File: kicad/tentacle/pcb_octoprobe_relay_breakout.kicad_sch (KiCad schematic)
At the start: 2 parts, among them J501 Conn_01x20, J502 Conn_01x20

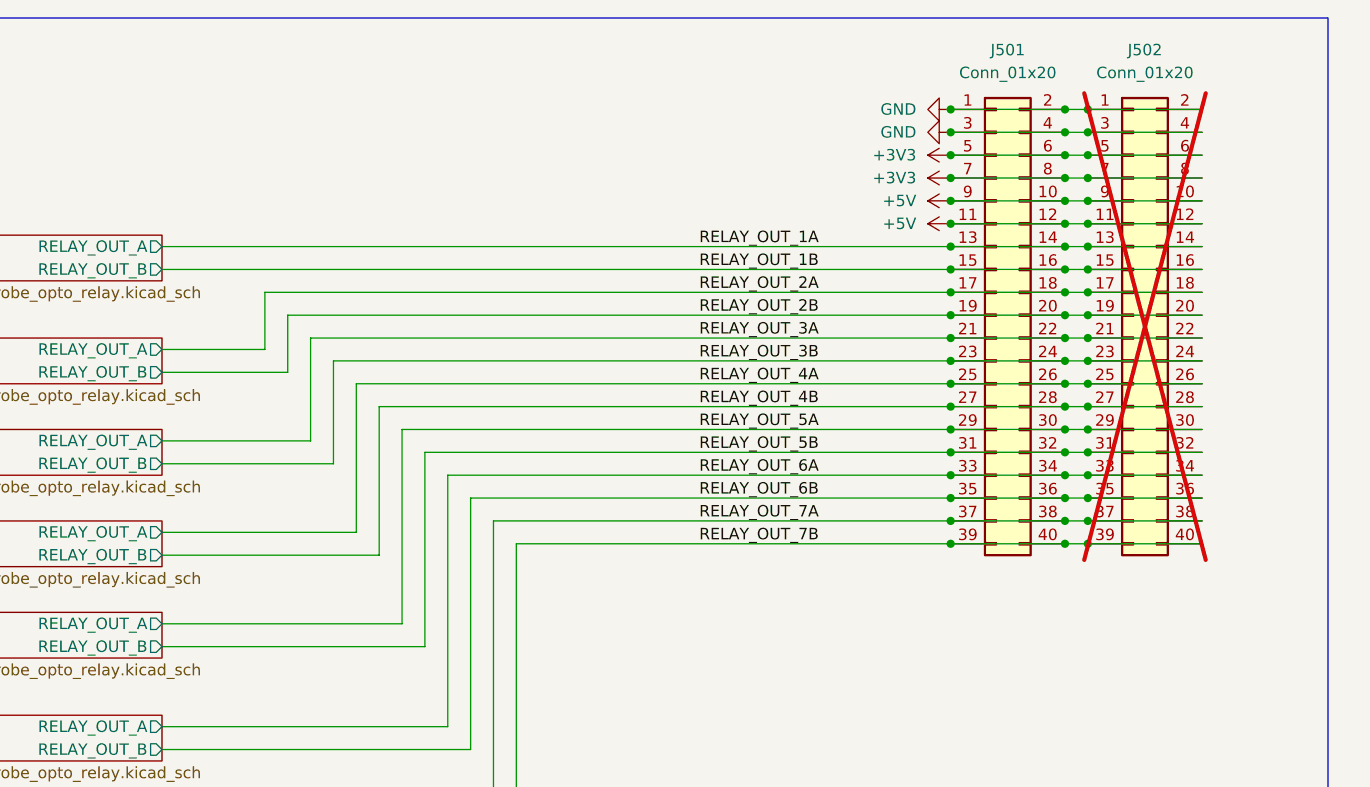
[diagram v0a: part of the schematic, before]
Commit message: Tentacle v0.4
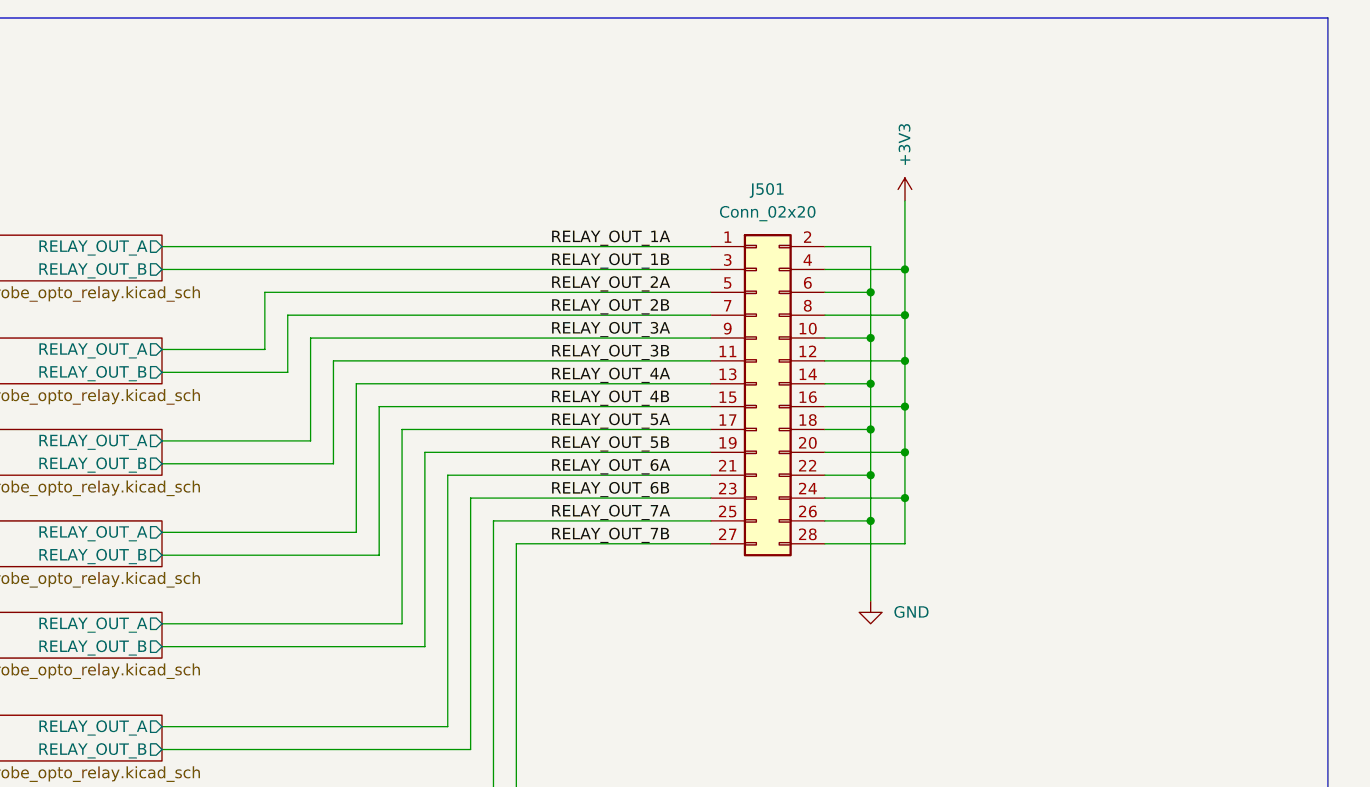
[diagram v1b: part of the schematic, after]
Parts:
- removed J501, J502: Conn_01x20, 00_project_library:PinSocket_2x20_P2.54mm_Vertical_squarepad, symbol Connector_Generic:Conn_02x20_Odd_Even
- added J501: Conn_02x20, 00_project_library:PinSocket_2x14_P2.54mm_Vertical_squarepad, symbol Connector_Generic:Conn_02x14_Odd_Even
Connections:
- net +3V3: now also J501.12 (Pin_12), J501.16 (Pin_16), J501.20 (Pin_20), J501.24 (Pin_24), J501.28 (Pin_28), J501.4 (Pin_4), J501.8 (Pin_8)
- net GND: now also J501.10 (Pin_10), J501.14 (Pin_14), J501.18 (Pin_18), J501.2 (Pin_2), J501.22 (Pin_22), J501.26 (Pin_26), J501.6 (Pin_6)
- net RELAY_OUT_1A: now also J501.1 (Pin_1)
- net RELAY_OUT_1B: now also J501.3 (Pin_3)
- net RELAY_OUT_2A: now also J501.5 (Pin_5)
- net RELAY_OUT_2B: now also J501.7 (Pin_7)
- net RELAY_OUT_3A: now also J501.9 (Pin_9)
- net RELAY_OUT_3B: now also J501.11 (Pin_11)
- net RELAY_OUT_4A: now also J501.13 (Pin_13)
- net RELAY_OUT_4B: now also J501.15 (Pin_15)
- net RELAY_OUT_5A: now also J501.17 (Pin_17)
- net RELAY_OUT_5B: now also J501.19 (Pin_19)
- net RELAY_OUT_6A: now also J501.21 (Pin_21)
- net RELAY_OUT_6B: now also J501.23 (Pin_23)
- net RELAY_OUT_7A: now also J501.25 (Pin_25)
- net RELAY_OUT_7B: now also J501.27 (Pin_27)
